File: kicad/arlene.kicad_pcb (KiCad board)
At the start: 2 copper layers, 81 x 46 mm, 97 parts, among them J1 24v, J2 Display, J3 Debug, J4 Handle, J5 USB-C, J6 Remote, Q1 AO4407, Q2 BC847, Q3 BC857, Q4 BC847, SW1 Encoder, U1 ACT4088, U2 LP5907-3.3, U3 STM32F072C8Tx, U4 MCP602, U5 MCP602, U6 SRV05-4

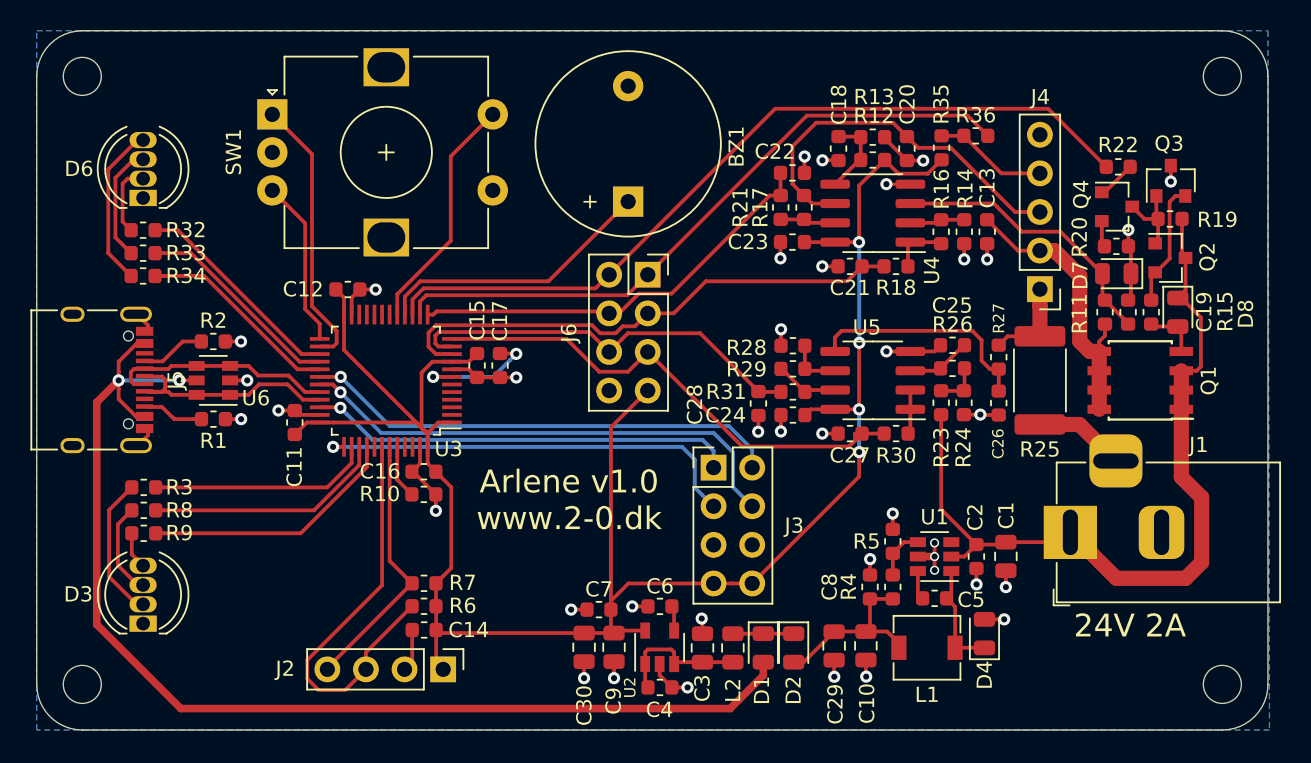
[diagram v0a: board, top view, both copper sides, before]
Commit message: Arlene v1.00
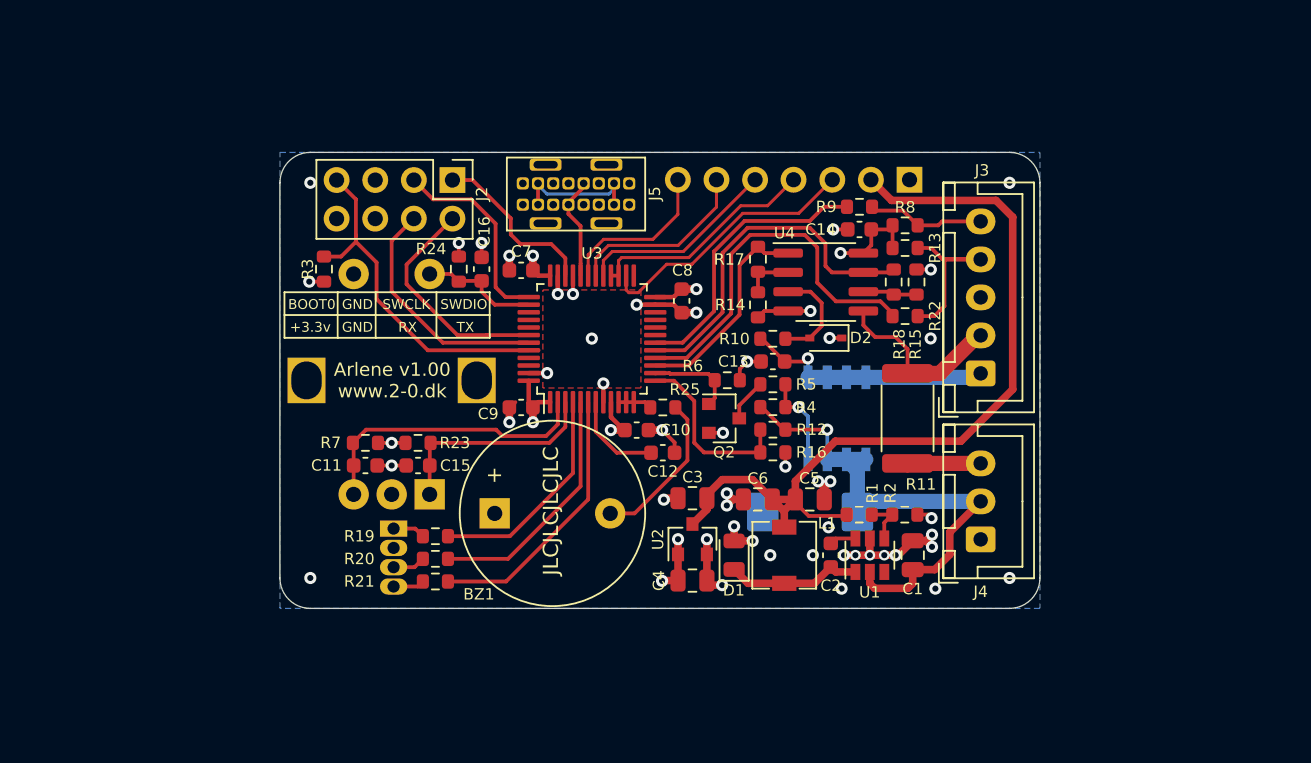
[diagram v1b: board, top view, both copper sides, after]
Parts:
- removed C18: 1u, Capacitor_SMD:C_0603_1608Metric
- removed C19, C20, C21, C22, C25, C26, C27, C28: nm, Capacitor_SMD:C_0603_1608Metric
- removed C23, C24: 100n, Capacitor_SMD:C_0603_1608Metric
- removed C29, C30: 10u, Capacitor_SMD:C_0805_2012Metric
- removed D4: 1N5819, Diode_SMD:D_0805_2012Metric
- removed D6: LED_CRGB, LED_THT:LED_D5.0mm-4_RGB
- removed D7: 1N4148, Diode_SMD:D_0805_2012Metric
- removed D8: 20v, Diode_SMD:D_0805_2012Metric
- removed H1, H2, H3, H4: MountingHole, MountingHole:MountingHole_2.5mm
- removed J6: Remote, Connector_PinSocket_2.54mm:PinSocket_2x04_P2.54mm_Vertical
- removed L2: Ferrite, Inductor_SMD:L_0805_2012Metric
- removed Q3: BC857, Package_TO_SOT_SMD:SOT-23
- removed Q4: BC847, Package_TO_SOT_SMD:SOT-23
- removed R26, R27, R29, R36: 10k, Resistor_SMD:R_0603_1608Metric
- removed R28: 1k, Resistor_SMD:R_0603_1608Metric
- removed R30, R31: 470, Resistor_SMD:R_0603_1608Metric
- removed R32, R33, R34: R, Resistor_SMD:R_0603_1608Metric
- removed R35: 4k7, Resistor_SMD:R_0603_1608Metric
- removed U5: MCP602, Package_SO:SOIC-8_3.9x4.9mm_P1.27mm
- removed U6: SRV05-4, Package_TO_SOT_SMD:SOT-23-6
- C10, C9: value 10u -> 100n; footprint Capacitor_SMD:C_0805_2012Metric -> Capacitor_SMD:C_0603_1608Metric
- C11, C15, C16: value 100n -> 1n
- C17: value 100n -> 100u; footprint Capacitor_SMD:C_0603_1608Metric -> Capacitor_Tantalum_SMD:CP_EIA-7343-31_Kemet-D; moved to B.Cu
- C2: value 100n -> 22n
- C4: value 100n -> 10u; footprint Capacitor_SMD:C_0603_1608Metric -> Capacitor_SMD:C_0805_2012Metric
- C5: value 22n -> 10u; footprint Capacitor_SMD:C_0603_1608Metric -> Capacitor_SMD:C_0805_2012Metric
- C6: value nm -> 10u; footprint Capacitor_SMD:C_0603_1608Metric -> Capacitor_SMD:C_0805_2012Metric
- D1: value D_Schottky -> 1N5819
- D2: value D_Schottky -> 1N4148; footprint Diode_SMD:D_0805_2012Metric -> Diode_SMD:D_SOD-323
- D3: value LED_CRGB -> LED_RCGB; footprint LED_THT:LED_D5.0mm-4_RGB -> arlene:LED_D5.0mm-4_RGB; moved to B.Cu
- J1: value 24v -> Display; footprint Connector_BarrelJack:BarrelJack_Horizontal -> Connector_PinHeader_2.54mm:PinHeader_1x07_P2.54mm_Vertical; moved to B.Cu
- J2: value Display -> Debug; footprint Connector_PinHeader_2.54mm:PinHeader_1x04_P2.54mm_Vertical -> Connector_PinHeader_2.54mm:PinHeader_2x04_P2.54mm_Vertical
- J3: value Debug -> Handle; footprint Connector_PinHeader_2.54mm:PinHeader_2x04_P2.54mm_Vertical -> Connector_JST:JST_XH_B5B-XH-A_1x05_P2.50mm_Vertical
- J4: value Handle -> Power; footprint Connector_PinHeader_2.54mm:PinHeader_1x05_P2.54mm_Vertical -> Connector_JST:JST_XH_B3B-XH-A_1x03_P2.50mm_Vertical
- J5: footprint Connector_USB:USB_C_Receptacle_XKB_U262-16XN-4BVC11 -> arlene:usb-c_14pin_tht_vertical
- L1: footprint arlene:L_4x4_H1.75 -> arlene:L_4.1x4.1_H1.75
- Q1: moved to B.Cu
- Q2: value BC847 -> AO3400A
- R1: value 5k1 -> 49.9k
- R10: value 100k -> 10k
- R11: value 10k -> 0.1; footprint Resistor_SMD:R_0603_1608Metric -> Resistor_SMD:R_2512_6332Metric
- R12: value 56k -> 10k
- R14: value 1k -> 1k1
- R15: value 100 -> 1k
- R16: value 150k -> 1k
- R17: value 14k -> 300k
- R18: value 470 -> 10k
- R19: value 5.1k -> 1k
- R2: value 5k1 -> 9.53k
- R21: value 470 -> 1k
- R22: value 100 -> 10k
- R23: value 6k8 -> 4k7
- R24: value 1k -> 4k7
- R25: value 0.1 -> 100; footprint Resistor_SMD:R_2512_6332Metric -> Resistor_SMD:R_0603_1608Metric
- R3: value R -> 100k
- R4: value 49.9k -> 10k
- R5: value 9.53k -> 2k
- R6: value 4k7 -> 100k
- R8, R9: value R -> 10k
- SW1: footprint Rotary_Encoder:RotaryEncoder_Alps_EC12E-Switch_Vertical_H20mm -> arlene:RotaryEncoder_Alps_EC12E-Switch_Vertical_H20mm; moved to B.Cu
- U2: value LP5907-3.3 -> XC6206PxxxMR; footprint Package_TO_SOT_SMD:SOT-23-5 -> Package_TO_SOT_SMD:SOT-23
- moved R8 53.5 mm to (166.1, 89.8), turned to 0 degrees
- moved R19 52.6 mm to (135.2, 110.2), turned to 0 degrees
- moved R9 51.8 mm to (163.1, 88.6), turned to 0 degrees
- moved R20 49.3 mm to (135.2, 111.7)
- moved R2 46.9 mm to (166.1, 108.8), turned to 0 degrees
- moved R1 42.9 mm to (163.1, 108.8), turned to 0 degrees
- moved C14 38.9 mm to (163.1, 90.1), turned to 0 degrees
- moved R23 34.5 mm to (134.1, 104.1), turned to 0 degrees
- moved R24 34.4 mm to (136.8, 92.7)
- moved J5 34.3 mm to (144.5, 87.7), turned to 0 degrees
- moved R21 33.5 mm to (135.2, 113.2), turned to 0 degrees
- moved J2 32.2 mm to (136.3, 86.8)
- moved Q2 31.2 mm to (154.2, 102.5)
- moved SW1 27.1 mm to (134.8, 107.5), turned to 90 degrees
- moved J1 25.5 mm to (166.4, 86.8), turned to 90 degrees
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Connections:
- BZ1 pad 1: hmi_buzzer -> +3V3
- BZ1 pad 2: GND -> Net-(BZ1-Pad2)
- C10 pad 1: switch_5v -> +3V3
- C11 pad 1: +3V3 -> enc_b
- C12 pad 1: +3V3 -> nrst
- C14 pad 1: +3V3 -> GND
- C14 pad 2: GND -> +3V3
- C15 pad 1: +3V3 -> GND
- C15 pad 2: GND -> enc_a
- C16 pad 1: +3V3 -> enc_switch
- C17 pad 1: nrst -> vin
- C2 pad 1: vin -> Net-(C2-Pad1)
- C2 pad 2: GND -> Net-(C2-Pad2)
- C3 pad 1: Net-(C3-Pad1) -> +5V
- C4 pad 1: Net-(C3-Pad1) -> +3V3
- C5 pad 1: Net-(C5-Pad1) -> +5V
- C5 pad 2: Net-(C5-Pad2) -> GND
- C6 pad 1: Net-(C6-Pad1) -> +5V
- C8 pad 1: switch_5v -> +3V3
- D1 pad 1: Net-(D1-Pad1) -> Net-(C2-Pad2)
- D1 pad 2: usb_vbus -> GND
- D2 pad 1: Net-(D1-Pad1) -> GND
- D2 pad 2: switch_5v -> Net-(D2-Pad2)
- D3 pad 1: GND -> Net-(D3-Pad1)
- D3 pad 2: Net-(D3-Pad2) -> GND
- J1 pad 1: vin -> GND
- J1 pad 2: GND -> +5V
- J1 pad 3: GND -> oled_sck
- J2 pad 1: +3V3 -> swdio
- J2 pad 2: GND -> uart_tx
- J2 pad 3: i2c_scl -> swclk
- J2 pad 4: i2c_sda -> uart_rx
- J3 pad 1: swdio -> pos_heater
- J3 pad 2: uart_tx -> neg_heater
- J3 pad 3: swclk -> Earth
- J3 pad 4: uart_rx -> handle_temperature
- J3 pad 5: GND -> handle_switch
- J4 pad 1: neg_heater -> Earth
- J4 pad 2: pos_heater -> vin
- J4 pad 3: thermistor -> GND
- J5 pad A4: usb_vbus -> Net-(J5-PadA4)
- J5 pad A5: Net-(J5-PadA5) -> (no net)
- J5 pad A9: usb_vbus -> Net-(J5-PadA4)
- J5 pad B4: usb_vbus -> Net-(J5-PadA4)
- J5 pad B5: Net-(J5-PadB5) -> (no net)
- J5 pad B9: usb_vbus -> Net-(J5-PadA4)
- J5 pad S1: GND -> Net-(J5-PadS1)
- L1 pad 1: Net-(C5-Pad2) -> Net-(C2-Pad2)
- L1 pad 2: switch_5v -> +5V
- Q1 pad 2: Net-(D8-Pad2) -> Net-(Q1-Pad2)
- Q2 pad 1: Net-(Q2-Pad1) -> pwm_heater
- Q2 pad 2: Net-(Q2-Pad2) -> GND
- Q2 pad 3: vin -> Net-(Q2-Pad3)
- R1 pad 1: GND -> +5V
- R1 pad 2: Net-(J5-PadB5) -> Net-(R1-Pad2)
- R10 pad 1: boot0 -> pos_heater
- R10 pad 2: GND -> Net-(D2-Pad2)
- R11 pad 1: pos_heater -> GND
- R11 pad 2: Net-(C19-Pad2) -> neg_heater
- R12 pad 1: Net-(C18-Pad2) -> adc_heater_voltage
- R12 pad 2: +3V3 -> vin
- R13 pad 1: GND -> handle_temperature
- R13 pad 2: Net-(C18-Pad2) -> +3V3
- R15 pad 1: Net-(Q2-Pad2) -> GND
- R15 pad 2: Net-(D8-Pad2) -> Net-(R15-Pad2)
- R16 pad 1: Net-(R14-Pad2) -> GND
- R16 pad 2: Net-(R16-Pad2) -> adc_heater_voltage
- R17 pad 1: thermistor -> Net-(R14-Pad2)
- R17 pad 2: Net-(R17-Pad2) -> adc_heater_temperature
- R18 pad 1: adc_heater_temp -> adc_heater_current
- R18 pad 2: Net-(R16-Pad2) -> Net-(R15-Pad2)
- R19 pad 1: vin -> Net-(D3-Pad1)
- R19 pad 2: Net-(Q2-Pad1) -> led_red
- R2 pad 1: GND -> Net-(R1-Pad2)
- R2 pad 2: Net-(J5-PadA5) -> GND
- R20 pad 1: Net-(Q4-Pad2) -> Net-(D3-Pad3)
- R20 pad 2: GND -> led_green
- R21 pad 1: adc_thermistor_temp -> Net-(D3-Pad4)
- R21 pad 2: Net-(R17-Pad2) -> led_blue
- R22 pad 1: pwm_heater -> adc_handle_temperature
- R22 pad 2: Net-(Q4-Pad1) -> handle_temperature
- R23 pad 1: Net-(R23-Pad1) -> +3V3
- R23 pad 2: vin -> enc_a
- R24 pad 1: GND -> enc_switch
- R24 pad 2: Net-(R23-Pad1) -> +3V3
- R25 pad 1: GND -> hmi_buzzer
- R25 pad 2: neg_heater -> Net-(BZ1-Pad2)
- R3 pad 1: led1_red -> boot0
- R3 pad 2: Net-(D3-Pad2) -> GND
- R4 pad 1: switch_5v -> vin
- R4 pad 2: Net-(R4-Pad2) -> Net-(Q1-Pad2)
- R5 pad 1: Net-(R4-Pad2) -> Net-(Q1-Pad2)
- R5 pad 2: GND -> Net-(Q2-Pad3)
- R6 pad 1: i2c_scl -> pwm_heater
- R6 pad 2: +3V3 -> GND
- R7 pad 1: i2c_sda -> enc_b
- R8 pad 1: led1_green -> +3V3
- R8 pad 2: Net-(D3-Pad3) -> handle_switch
- R9 pad 1: led1_blue -> handle_switch_in
- R9 pad 2: Net-(D3-Pad4) -> handle_switch
- U1 pad 1: Net-(C5-Pad2) -> Net-(C2-Pad2)
- U1 pad 4: Net-(R4-Pad2) -> Net-(R1-Pad2)
- U1 pad 6: Net-(C5-Pad1) -> Net-(C2-Pad1)
- U2 pad 1: Net-(C3-Pad1) -> GND
- U2 pad 2: GND -> +3V3
- U2 pad 3: Net-(C3-Pad1) -> +5V
- U3 pad 10: adc_heater_temp -> hmi_buzzer
- U3 pad 11: adc_current -> hmi_buzzer
- U3 pad 12: adc_voltage -> hmi_buzzer
- U3 pad 13: adc_thermistor_temp -> adc_heater_voltage
- U3 pad 14: handle_switch -> pwm_heater
- U3 pad 15: pwm_heater -> adc_heater_temperature
- U3 pad 16: hmi_buzzer -> adc_handle_temperature
- U3 pad 17: enc_switch -> adc_heater_current
- U3 pad 18: (no net) -> handle_switch_in
- U3 pad 2: (no net) -> enc_b
- U3 pad 25: enc_b -> (no net)
- U3 pad 26: enc_a -> oled_sck
- U3 pad 27: led2_red -> oled_sda
- U3 pad 28: led2_green -> oled_sda
- U3 pad 29: led2_blue -> oled_reset
- U3 pad 3: (no net) -> enc_a
- U3 pad 30: uart_tx -> oled_dc
- U3 pad 31: uart_rx -> oled_cs
- U3 pad 38: led1_red -> enc_switch
- U3 pad 39: led1_green -> (no net)
- U3 pad 4: (no net) -> led_red
- U3 pad 40: led1_blue -> (no net)
- U3 pad 42: i2c_scl -> uart_tx
- U3 pad 43: i2c_sda -> uart_rx
- U3 pad 5: (no net) -> led_green
- U3 pad 6: (no net) -> led_blue
- U4 pad 1: Net-(R16-Pad2) -> adc_heater_temperature
- U4 pad 3: Net-(C19-Pad2) -> Net-(D2-Pad2)
- U4 pad 5: Net-(C18-Pad2) -> neg_heater
- U4 pad 6: thermistor -> Net-(R15-Pad2)
- U4 pad 7: Net-(R17-Pad2) -> adc_heater_current
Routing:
- net +3V3: track 134.3 -> 25.2 mm, vias 4 -> 9
- net usb_vbus: track 77.0 -> 0.00 mm, vias 2 -> 0
- net +5V: track 0.00 -> 57.1 mm
- net pwm_heater: track 53.4 -> 5.86 mm
- net handle_switch: track 43.8 -> 7.87 mm
- net adc_heater_temp: track 34.9 -> 0.00 mm
- net adc_voltage: track 33.1 -> 0.00 mm
- net adc_thermistor_temp: track 28.1 -> 0.00 mm
- net i2c_scl: track 27.4 -> 0.00 mm
- net adc_current: track 27.2 -> 0.00 mm
- net thermistor: track 25.2 -> 0.00 mm
- net adc_handle_temperature: track 0.00 -> 24.9 mm
- net GND: track 76.3 -> 51.6 mm, vias 39 -> 46
- net adc_heater_current: track 0.00 -> 23.5 mm
- net vin: track 53.7 -> 33.6 mm, vias 0 -> 1
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- added copper zone on In2.Cu, net +3V3
- added copper zone on F.Cu, net GND
- added copper zone on In1.Cu, net GND
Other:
- board size 81 x 46 mm -> 50 x 30 mm
- copper layers 2 -> 4
- rule pad_to_mask_clearance: 0.051 -> 0
- board text added: "+24v"
- board text added: "+3.3v"
- board text added: "Arlene v1.00 www.2-0.dk"
- board text added: "BOOT0"
- board text added: "Earth"
- board text added: "GND"
- board text added: "Handle"
- board text added: "Heater+"
- board text added: "Heater-"
- board text added: "JLCJLCJLCJLC"
- board text added: "NTC"
- board text added: "OLED"
- board text added: "Power"
- board text added: "RX"
- board text added: "SWCLK"
- board text added: "SWDIO"
- board text added: "Switch"
- board text added: "TX"
- board text removed: "24V 2A"
- board text removed: "Arlene v1.0 www.2-0.dk"
